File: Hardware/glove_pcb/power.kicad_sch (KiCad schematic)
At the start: 7 parts, among them J2 Barrel_Jack_Switch

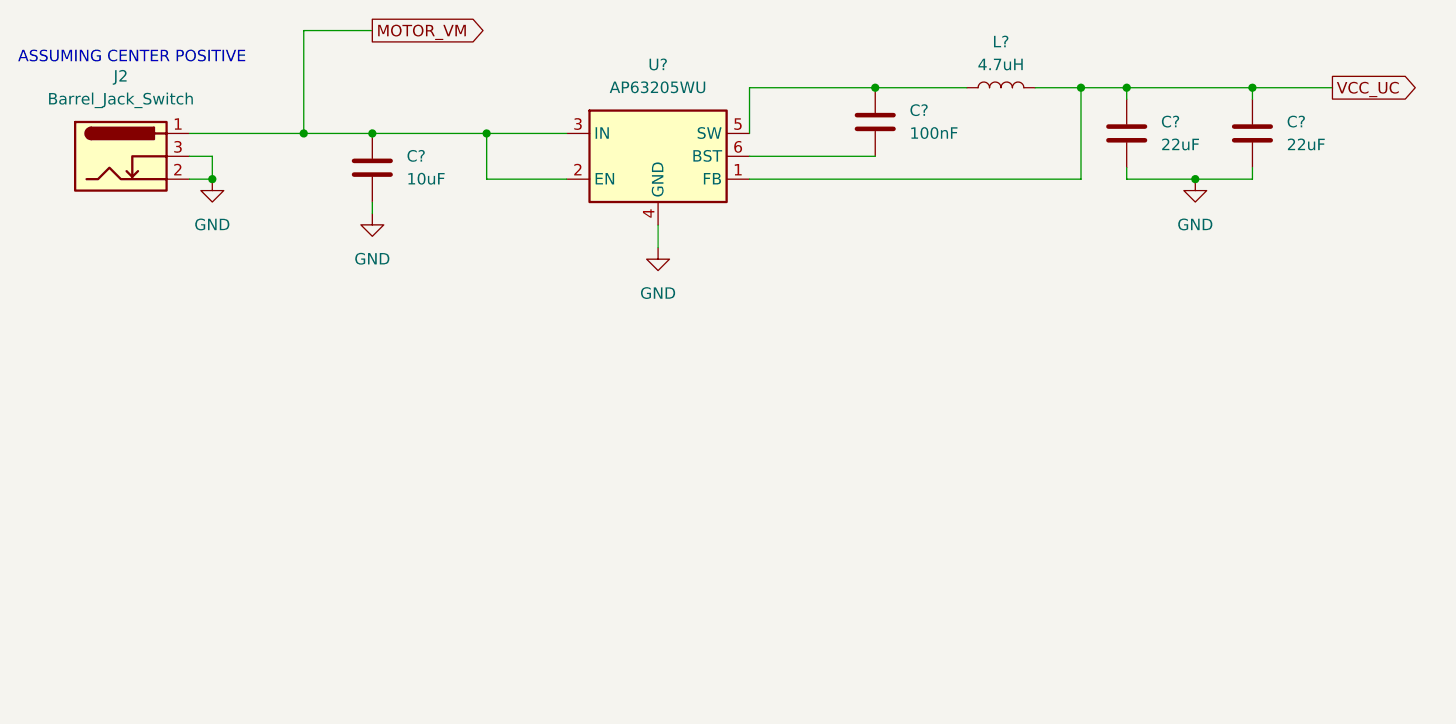
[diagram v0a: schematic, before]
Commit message: Finish controller pin assignments
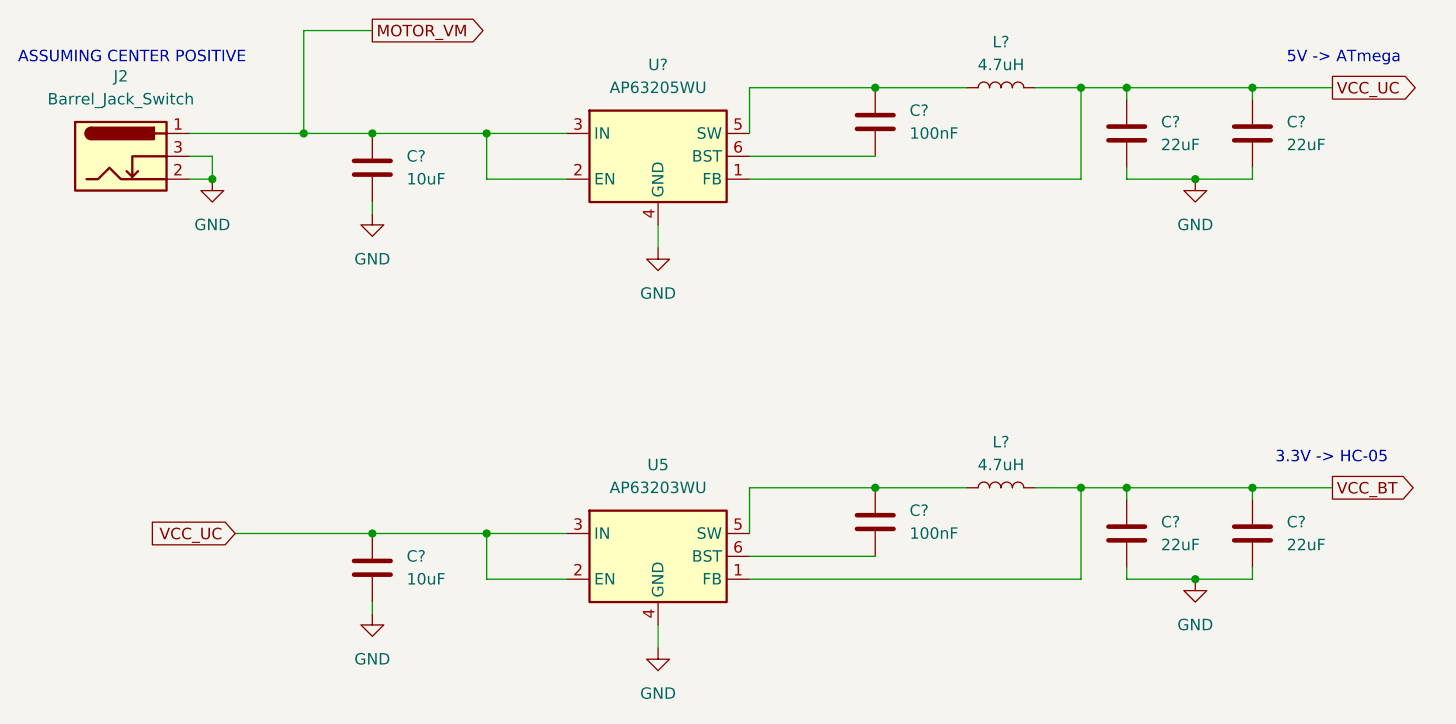
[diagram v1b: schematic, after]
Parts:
- added C?: 100nF, symbol Device:C
- added C? (x2): 22uF, symbol Device:C
- added C?: 10uF, symbol Device:C
- added L?: 4.7uH, symbol Device:L
- added U5: AP63203WU, Package_TO_SOT_SMD:TSOT-23-6, symbol Regulator_Switching:AP63203WU
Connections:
- net GND: now also C?.2, C?.2, C?.2, U5.4 (GND)
- net VCC_UC: now also C?.1, U5.2 (EN), U5.3 (IN)
- new net: C?.1, L?.1, U5.5 (SW)
- new net: C?.2, U5.6 (BST)
- new net VCC_BT: C?.1, C?.1, L?.2, U5.1 (FB)
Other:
- note added: "3.3V -> HC-05"
- note added: "5V -> ATmega"
